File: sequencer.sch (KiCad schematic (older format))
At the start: 196 parts, among them IC1 ATMEGA328PB, IC2 AT24CS64-XHM, J13 SYNC IN, J14 TRIGGER OUT 1, J15 TRIGGER OUT 2, P12 CONN_01X03, P3 CONN_02X10, P6 CONN_01X03, P7 CONN_02X03, Q38 C945, Q64 C945, Q75 A733, SW10 INST_CH_12, SW11 SHIFT, SW12 IF_VAR, SW13 INST_LT_4, SW14 INST_MT_5, SW15 INST_HT_6, SW16 INST_RS_7, SW17 INST_CP_8, SW18 INST_CB_9, SW19 INST_CY_10, SW2 BASIC_VAR_A, SW20 INST_OH_11, SW21 START/STOP, SW22 TAP, SW4 MODE, SW5 FILL, SW6 CLEAR, SW7 INST_AC_1, SW8 INST_BD_2, SW9 INST_SD_3, U27 74HC165, U28 74HC165, U29 74HC165, U30 74AC595, U31 74AC595, U32 74AC595, U33 74AC595, U34 74AC595, U35 R-78E5.0-1.0, U36 74AC595, U37 74AC595, X1 MIDI IN, Y1 16MHz

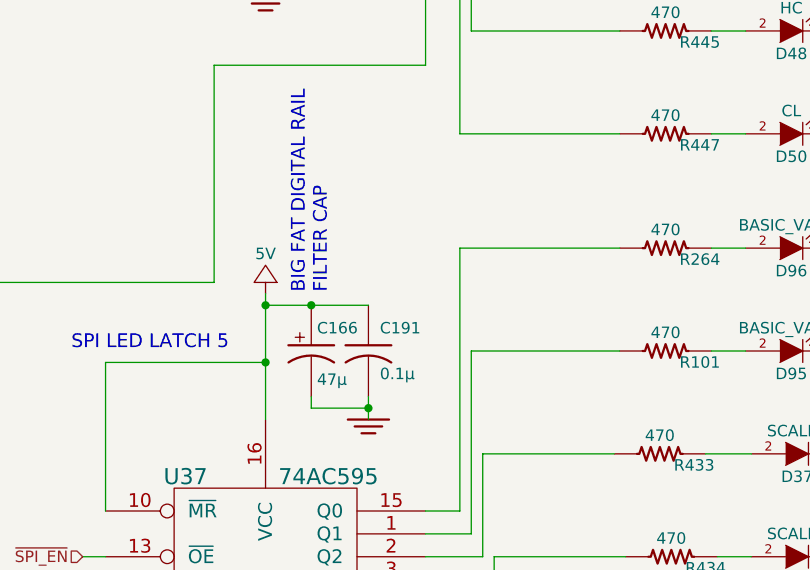
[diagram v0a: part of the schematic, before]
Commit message: few tweaks, ready to generate gerbers for 2.1 production prototype
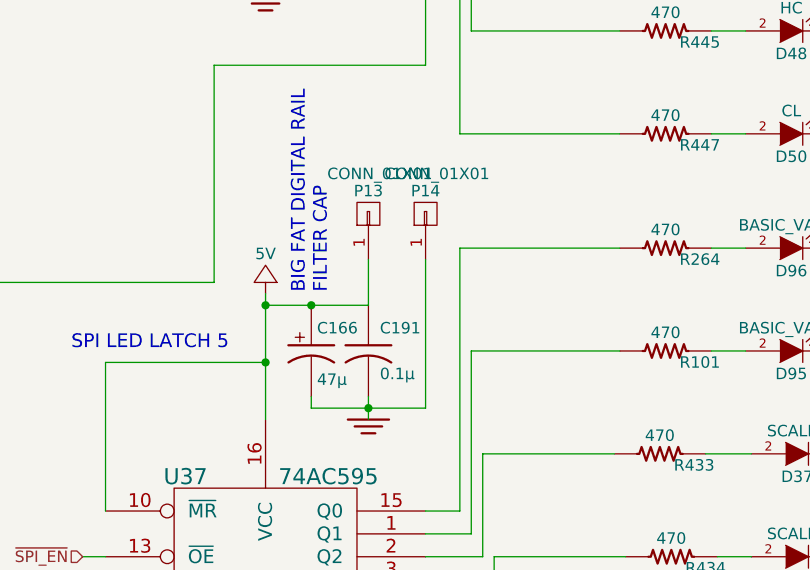
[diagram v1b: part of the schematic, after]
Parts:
- added P13, P14: CONN_01X01, MyModules:TEST_POINT_SMALL, symbol CONN_01X01
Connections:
- net +5V: now also P13.1 (P1)
- net GND: now also P14.1 (P1)
